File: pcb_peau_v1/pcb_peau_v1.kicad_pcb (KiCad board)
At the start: 2 copper layers, 72.1 x 71 mm, 25 parts, among them J1 Conn_01x05, J2 Conn_01x05, J4 Conn_02x08_Top_Bottom, J5 Conn_02x12_Top_Bottom, U2 TLC274, U3 CD74HC4067SM, U4 CD74HC4067SM, U5 CD74HC4067SM, U6 CD74HC4067SM, U7 TLC274, U8 TLC274, U9 TLC274

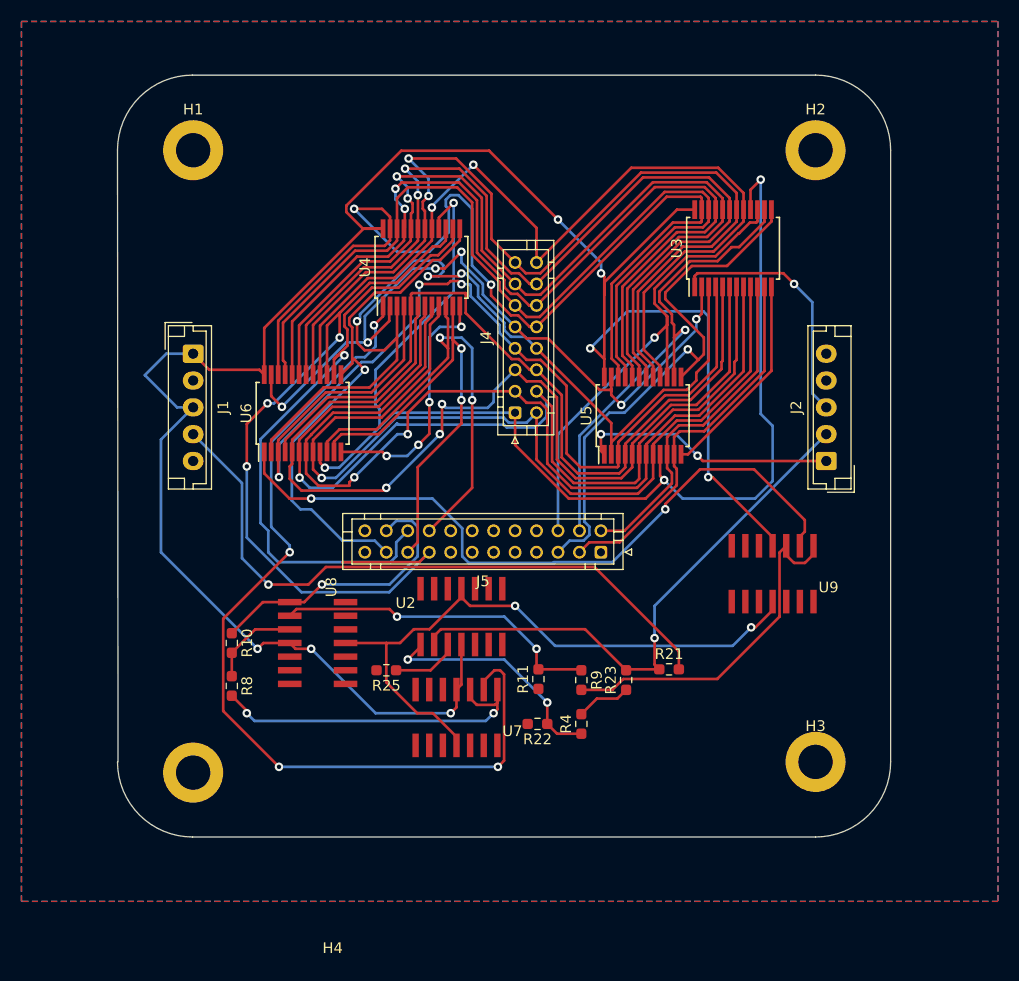
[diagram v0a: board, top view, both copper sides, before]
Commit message: PCB corrigé
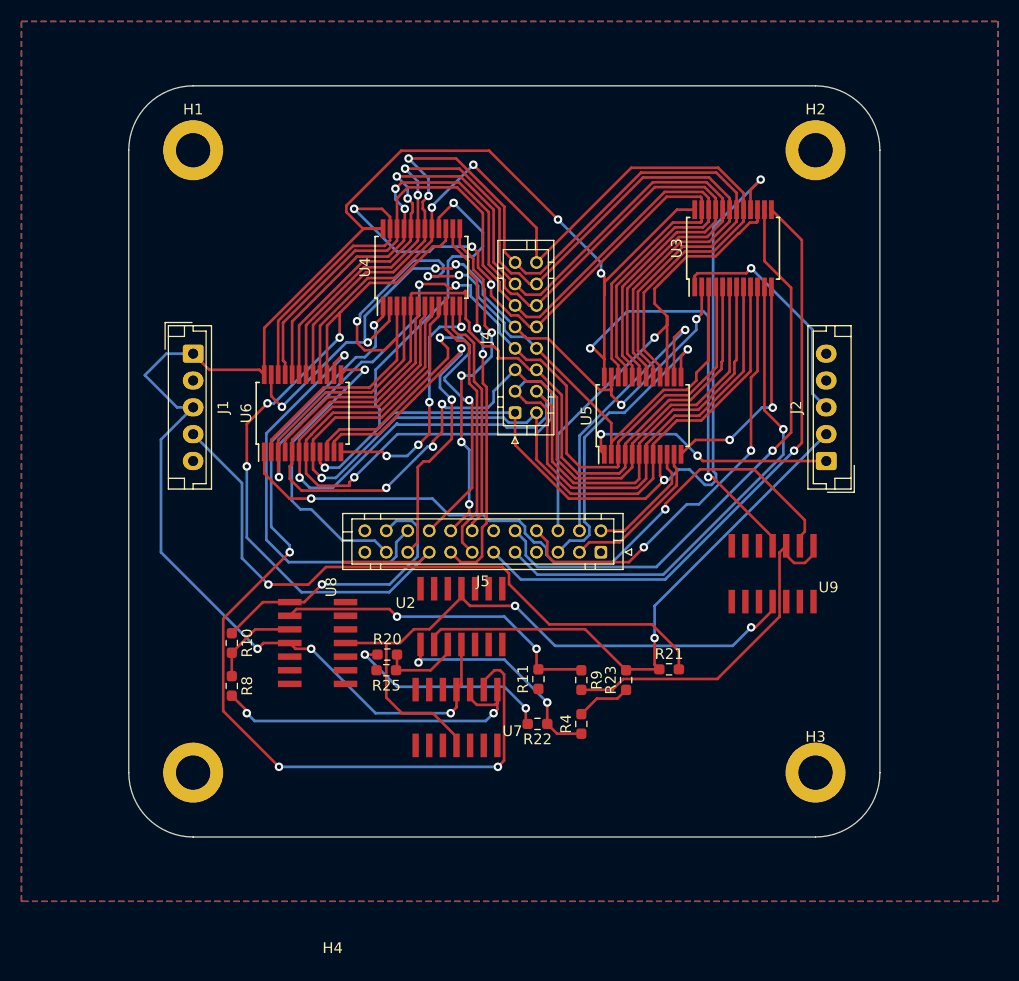
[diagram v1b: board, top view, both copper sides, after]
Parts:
- added R20: 1M, Resistor_SMD:R_0603_1608Metric_Pad0.98x0.95mm_HandSolder, F.Cu at (196.1, 100.0)
- moved H3 1.00 mm to (236.0, 111.0)
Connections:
- J5 pad 10: unconnected-(J5-Pin_10-Pad10) -> C3
- J5 pad 11: unconnected-(J5-Pin_11-Pad11) -> D3
- J5 pad 13: unconnected-(J5-Pin_13-Pad13) -> A4
- J5 pad 14: unconnected-(J5-Pin_14-Pad14) -> B4
- J5 pad 15: unconnected-(J5-Pin_15-Pad15) -> C4
- J5 pad 16: unconnected-(J5-Pin_16-Pad16) -> D4
- J5 pad 8: unconnected-(J5-Pin_8-Pad8) -> A3
- J5 pad 9: unconnected-(J5-Pin_9-Pad9) -> B3
- U3 pad 10: A1 -> A3
- U3 pad 11: B1 -> B3
- U3 pad 13: D1 -> D3
- U3 pad 14: C1 -> C3
- U4 pad 10: A2 -> A4
- U4 pad 11: B2 -> B4
- U4 pad 13: D2 -> D4
- U4 pad 14: C2 -> C4
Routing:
- net D3: track 0.00 -> 58.0 mm, vias 0 -> 1
- net C3: track 0.00 -> 54.9 mm, vias 0 -> 1
- net B3: track 0.00 -> 46.9 mm, vias 0 -> 1
- net A3: track 0.00 -> 41.9 mm, vias 0 -> 2
- net C4: track 0.00 -> 35.5 mm, vias 0 -> 2
- net D4: track 0.00 -> 32.2 mm, vias 0 -> 4
- net A4: track 0.00 -> 25.5 mm
- net B4: track 0.00 -> 22.8 mm
- net D1: track 51.3 -> 28.7 mm
- net B1: track 35.1 -> 14.6 mm
- net A1: track 31.8 -> 11.3 mm
- net C2: track 58.6 -> 38.6 mm
- net Net-(R20-Pad1): track 0.00 -> 19.8 mm, vias 0 -> 2
- net D2: track 47.6 -> 28.2 mm
- net C1: track 46.3 -> 27.8 mm
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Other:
- board size 72.1 x 71 mm -> 70 x 70 mm
